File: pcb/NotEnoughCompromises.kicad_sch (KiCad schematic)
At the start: 128 parts, among them J1 MJ-4PP-9, J2 MJ-4PP-9, SW1 SW_PUSH, SW10 SW_PUSH, SW11 SW_PUSH, SW12 SW_PUSH, SW13 SW_PUSH, SW14 SW_PUSH, SW15 SW_PUSH, SW16 SW_PUSH, SW17 SW_PUSH, SW18 SW_PUSH, SW19 SW_PUSH, SW2 SW_PUSH, SW20 SW_PUSH, SW21 SW_PUSH, SW22 SW_PUSH, SW23 SW_PUSH, SW24 RESET_SW, SW25 SW_PUSH, SW26 SW_PUSH, SW27 SW_PUSH, SW28 SW_PUSH, SW29 SW_PUSH, SW3 SW_PUSH, SW30 RESET_SW, SW31 SW_PUSH, SW32 SW_PUSH, SW33 SW_PUSH, SW34 SW_PUSH, SW35 SW_PUSH, SW36 SW_PUSH, SW37 SW_PUSH, SW38 SW_PUSH, SW39 SW_PUSH, SW4 SW_PUSH, SW40 SW_PUSH, SW41 SW_PUSH, SW42 SW_PUSH, SW43 SW_PUSH, SW44 SW_PUSH, SW45 SW_PUSH, SW46 SW_PUSH, SW47 SW_PUSH, SW48 SW_PUSH, SW49 SW_PUSH, SW5 SW_PUSH, SW50 SW_PUSH, SW51 SW_PUSH, SW52 SW_PUSH, SW53 SW_PUSH, SW54 SW_PUSH, SW55 SW_PUSH, SW56 SW_PUSH, SW57 SW_PUSH, SW58 SW_PUSH, SW6 SW_PUSH, SW7 SW_PUSH, SW8 SW_PUSH, SW9 SW_PUSH, U1 ProMicro, U2 ProMicro

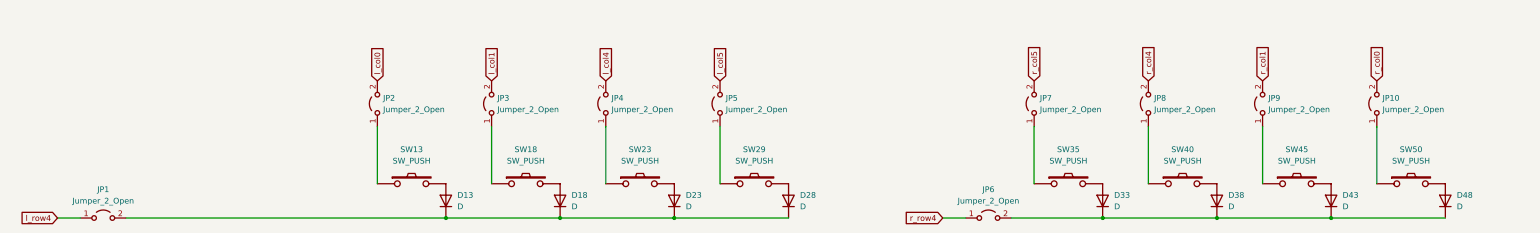
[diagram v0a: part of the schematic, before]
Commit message: 部品を配置した
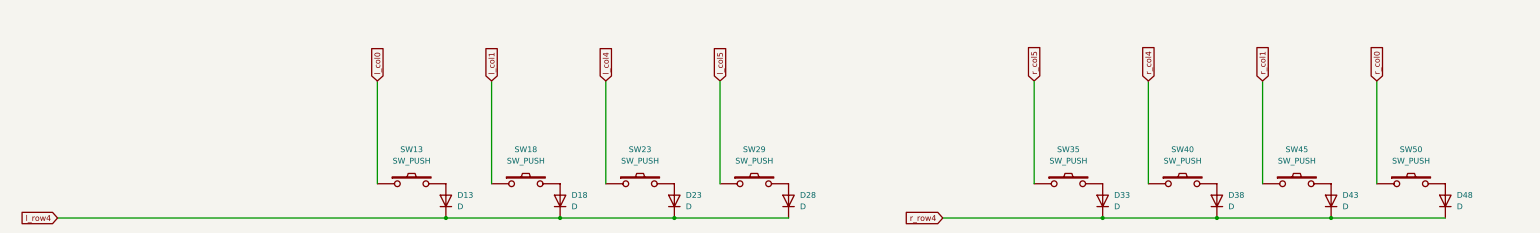
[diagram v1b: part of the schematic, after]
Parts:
- removed JP1, JP10, JP2, JP3, JP4, JP5, JP6, JP7, JP8, JP9: Jumper_2_Open, symbol Jumper:Jumper_2_Open
- D1, D10, D11, D12, D13, D14, D15, D16, D17, D18, D19, D2, D20, D21, D22, D23, D24, D25, D26, D27, D28, D29, D3, D30, D31, D32, D33, D34, D35, D36, D37, D38, D39, D4, D40, D41, D42, D43, D44, D45, D46, D47, D48, D49, D5, D50, D51, D52, D53, D54, D55, D56, D6, D7, D8, D9: footprint (none) -> kbd:D3_SMD_v2
- J1, J2: footprint (none) -> kbd:MJ-4PP-9_1side
- SW1, SW10, SW11, SW12, SW13, SW14, SW15, SW16, SW17, SW18, SW19, SW2, SW20, SW21, SW22, SW23, SW25, SW26, SW27, SW28, SW29, SW3, SW31, SW32, SW33, SW34, SW35, SW36, SW37, SW38, SW39, SW4, SW40, SW41, SW42, SW43, SW44, SW45, SW46, SW47, SW48, SW49, SW5, SW50, SW51, SW52, SW53, SW54, SW55, SW56, SW57, SW58, SW6, SW7, SW8, SW9: footprint (none) -> not_enough_compromises:choc_v1
- SW24, SW30: footprint (none) -> kbd:ResetSW_1side
- U1, U2: footprint (none) -> kbd:ProMicro_v3.5
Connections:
- net l_col0: now also SW13.1
- net l_col1: now also SW18.1
- net l_col4: now also SW23.1
- net l_col5: now also SW29.1
- net l_row4: now also D13.1 (K), D18.1 (K), D23.1 (K), D28.1 (K)
- net r_col0: now also SW50.1
- net r_col1: now also SW45.1
- net r_col4: now also SW40.1
- net r_col5: now also SW35.1
- net r_row4: now also D33.1 (K), D38.1 (K), D43.1 (K), D48.1 (K)

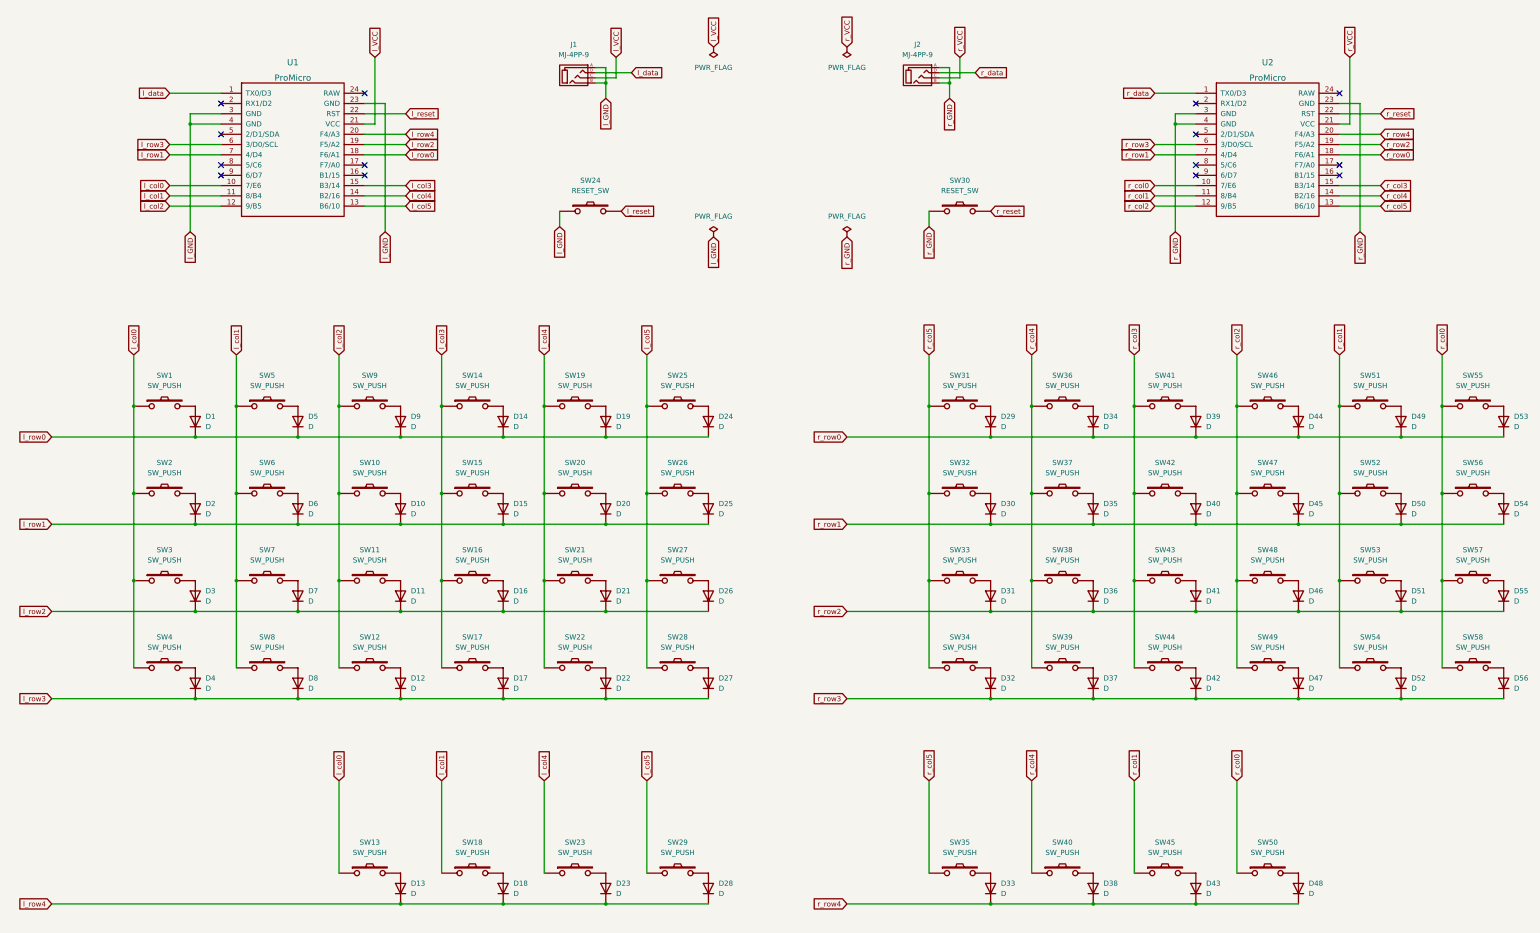
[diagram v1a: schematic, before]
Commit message: 基板を作成
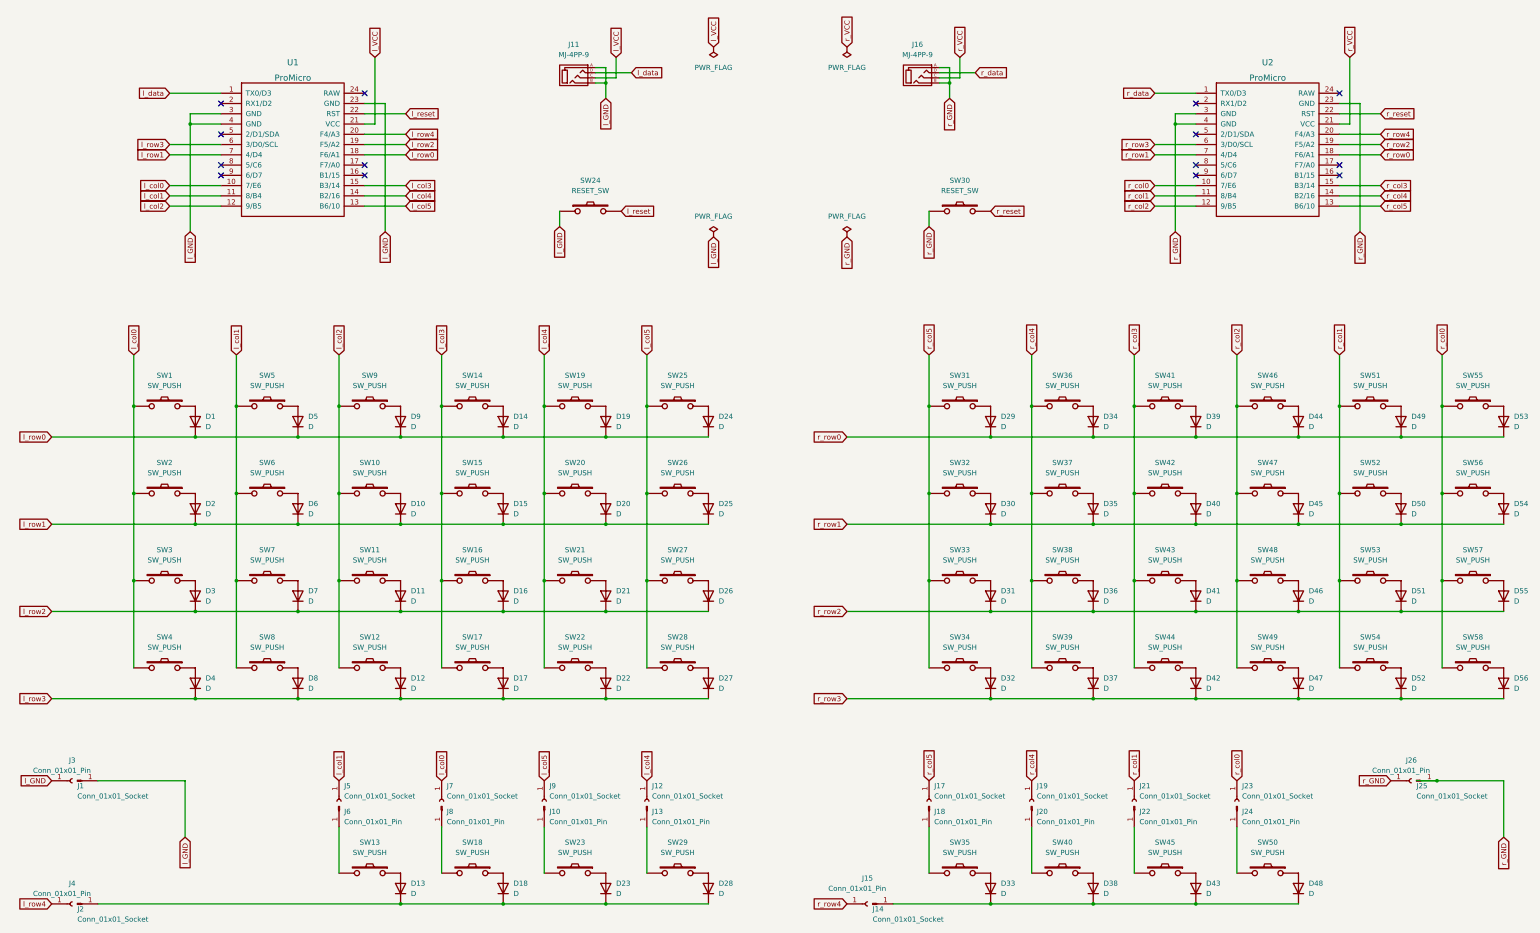
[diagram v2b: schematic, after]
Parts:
- added J1, J12, J14, J17, J19, J2, J21, J23, J25, J5, J7, J9: Conn_01x01_Socket, Connector_Wire:SolderWirePad_1x01_SMD_1x2mm, symbol Connector:Conn_01x01_Socket
- added J10, J13, J15, J18, J20, J22, J24, J26, J3, J4, J6, J8: Conn_01x01_Pin, Connector_Wire:SolderWirePad_1x01_SMD_1x2mm, symbol Connector:Conn_01x01_Pin
- SW24, SW30: footprint kbd:ResetSW_1side -> not_enough_compromises:reset_sw
- renumbered J1 to J11, J2 to J16
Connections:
- net l_GND: now also J1.1 (Pin_1), J3.1 (Pin_1)
- net l_col0: now also SW1.2, SW2.2, SW3.2, SW4.2, J7.1 (Pin_1); no longer SW1.1, SW13.1, SW2.1, SW3.1, SW4.1
- net l_col1: now also SW5.2, SW6.2, SW7.2, SW8.2, J5.1 (Pin_1); no longer SW18.1, SW5.1, SW6.1, SW7.1, SW8.1
- net l_col2: now also SW10.2, SW11.2, SW12.2, SW9.2; no longer SW10.1, SW11.1, SW12.1, SW9.1
- net l_col3: now also SW14.2, SW15.2, SW16.2, SW17.2; no longer SW14.1, SW15.1, SW16.1, SW17.1
- net l_col4: now also SW19.2, SW20.2, SW21.2, SW22.2, J12.1 (Pin_1); no longer SW19.1, SW20.1, SW21.1, SW22.1, SW23.1
- net l_col5: now also SW25.2, SW26.2, SW27.2, SW28.2, J9.1 (Pin_1); no longer SW25.1, SW26.1, SW27.1, SW28.1, SW29.1
- net l_row4: now also J2.1 (Pin_1); no longer D13.1 (K), D18.1 (K), D23.1 (K), D28.1 (K)
- net r_GND: now also J25.1 (Pin_1), J26.1 (Pin_1)
- net r_col0: now also SW55.2, SW56.2, SW57.2, SW58.2, J23.1 (Pin_1); no longer SW50.1, SW55.1, SW56.1, SW57.1, SW58.1
- net r_col1: now also SW51.2, SW52.2, SW53.2, SW54.2, J21.1 (Pin_1); no longer SW45.1, SW51.1, SW52.1, SW53.1, SW54.1
- net r_col2: now also SW46.2, SW47.2, SW48.2, SW49.2; no longer SW46.1, SW47.1, SW48.1, SW49.1
- net r_col3: now also SW41.2, SW42.2, SW43.2, SW44.2; no longer SW41.1, SW42.1, SW43.1, SW44.1
- net r_col4: now also SW36.2, SW37.2, SW38.2, SW39.2, J19.1 (Pin_1); no longer SW36.1, SW37.1, SW38.1, SW39.1, SW40.1
- net r_col5: now also SW31.2, SW32.2, SW33.2, SW34.2, J17.1 (Pin_1); no longer SW31.1, SW32.1, SW33.1, SW34.1, SW35.1
- net r_row4: now also J14.1 (Pin_1); no longer D33.1 (K), D38.1 (K), D43.1 (K), D48.1 (K)
- net at D12.2 (A): now also SW12.1; no longer SW12.2
- net at D36.2 (A): now also SW38.1; no longer SW38.2
- net at D41.2 (A): now also SW43.1; no longer SW43.2
- net at D47.2 (A): now also SW49.1; no longer SW49.2
- net at D27.2 (A): now also SW28.1; no longer SW28.2
- net at D23.2 (A): now also SW23.1; no longer SW23.2
- net at D22.2 (A): now also SW22.1; no longer SW22.2
- net at D19.2 (A): now also SW19.1; no longer SW19.2
- net at D39.2 (A): now also SW41.1; no longer SW41.2
- net at D54.2 (A): now also SW56.1; no longer SW56.2
- net at D56.2 (A): now also SW58.1; no longer SW58.2
- net at D26.2 (A): now also SW27.1; no longer SW27.2
- net at D30.2 (A): now also SW32.1; no longer SW32.2
- net at D40.2 (A): now also SW42.1; no longer SW42.2
- net at D45.2 (A): now also SW47.1; no longer SW47.2
- net at D42.2 (A): now also SW44.1; no longer SW44.2
- net at D38.2 (A): now also SW40.1; no longer SW40.2
- net at D11.2 (A): now also SW11.1; no longer SW11.2
- net at D46.2 (A): now also SW48.1; no longer SW48.2
- net at D29.2 (A): now also SW31.1; no longer SW31.2
- net at D34.2 (A): now also SW36.1; no longer SW36.2
- net at D6.2 (A): now also SW6.1; no longer SW6.2
- net at D4.2 (A): now also SW4.1; no longer SW4.2
- net at D10.2 (A): now also SW10.1; no longer SW10.2
- net at D16.2 (A): now also SW16.1; no longer SW16.2
- net at D1.2 (A): now also SW1.1; no longer SW1.2
- net at D24.2 (A): now also SW25.1; no longer SW25.2
- net at D5.2 (A): now also SW5.1; no longer SW5.2
- net at D25.2 (A): now also SW26.1; no longer SW26.2
- net at D9.2 (A): now also SW9.1; no longer SW9.2
- net at D50.2 (A): now also SW52.1; no longer SW52.2
- net at D35.2 (A): now also SW37.1; no longer SW37.2
- net at D13.2 (A): now also SW13.1; no longer SW13.2
- net at D21.2 (A): now also SW21.1; no longer SW21.2
- net at D15.2 (A): now also SW15.1; no longer SW15.2
- net at D53.2 (A): now also SW55.1; no longer SW55.2
- net at SW35.2: now also J18.1 (Pin_1); no longer D33.2 (A)
- net at D43.2 (A): now also SW45.1; no longer SW45.2
- net at D32.2 (A): now also SW34.1; no longer SW34.2
- net at D37.2 (A): now also SW39.1; no longer SW39.2
- net at D49.2 (A): now also SW51.1; no longer SW51.2
- net at D18.2 (A): now also SW18.1; no longer SW18.2
- net at D2.2 (A): now also SW2.1; no longer SW2.2
- net at SW50.2: now also J24.1 (Pin_1); no longer D48.2 (A)
- net at D28.2 (A): now also SW29.1; no longer SW29.2
- net at D51.2 (A): now also SW53.1; no longer SW53.2
- net at D20.2 (A): now also SW20.1; no longer SW20.2
- net at D55.2 (A): now also SW57.1; no longer SW57.2
- net at D7.2 (A): now also SW7.1; no longer SW7.2
- net at D52.2 (A): now also SW54.1; no longer SW54.2
- net at D3.2 (A): now also SW3.1; no longer SW3.2
- net at D14.2 (A): now also SW14.1; no longer SW14.2
- net at D8.2 (A): now also SW8.1; no longer SW8.2
- net at D17.2 (A): now also SW17.1; no longer SW17.2
- net at D31.2 (A): now also SW33.1; no longer SW33.2
- net at D44.2 (A): now also SW46.1; no longer SW46.2
- new net: D13.1 (K), D18.1 (K), D23.1 (K), D28.1 (K), J4.1 (Pin_1)
- new net: D33.1 (K), D38.1 (K), D43.1 (K), D48.1 (K), J15.1 (Pin_1)
- new net: J6.1 (Pin_1), SW13.2
- new net: D33.2 (A), SW35.1
- new net: J22.1 (Pin_1), SW45.2
- new net: J8.1 (Pin_1), SW18.2
- new net: D48.2 (A), SW50.1
- new net: J10.1 (Pin_1), SW23.2
- new net: J20.1 (Pin_1), SW40.2
- new net: J13.1 (Pin_1), SW29.2
